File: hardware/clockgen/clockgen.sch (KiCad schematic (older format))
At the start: 2 parts

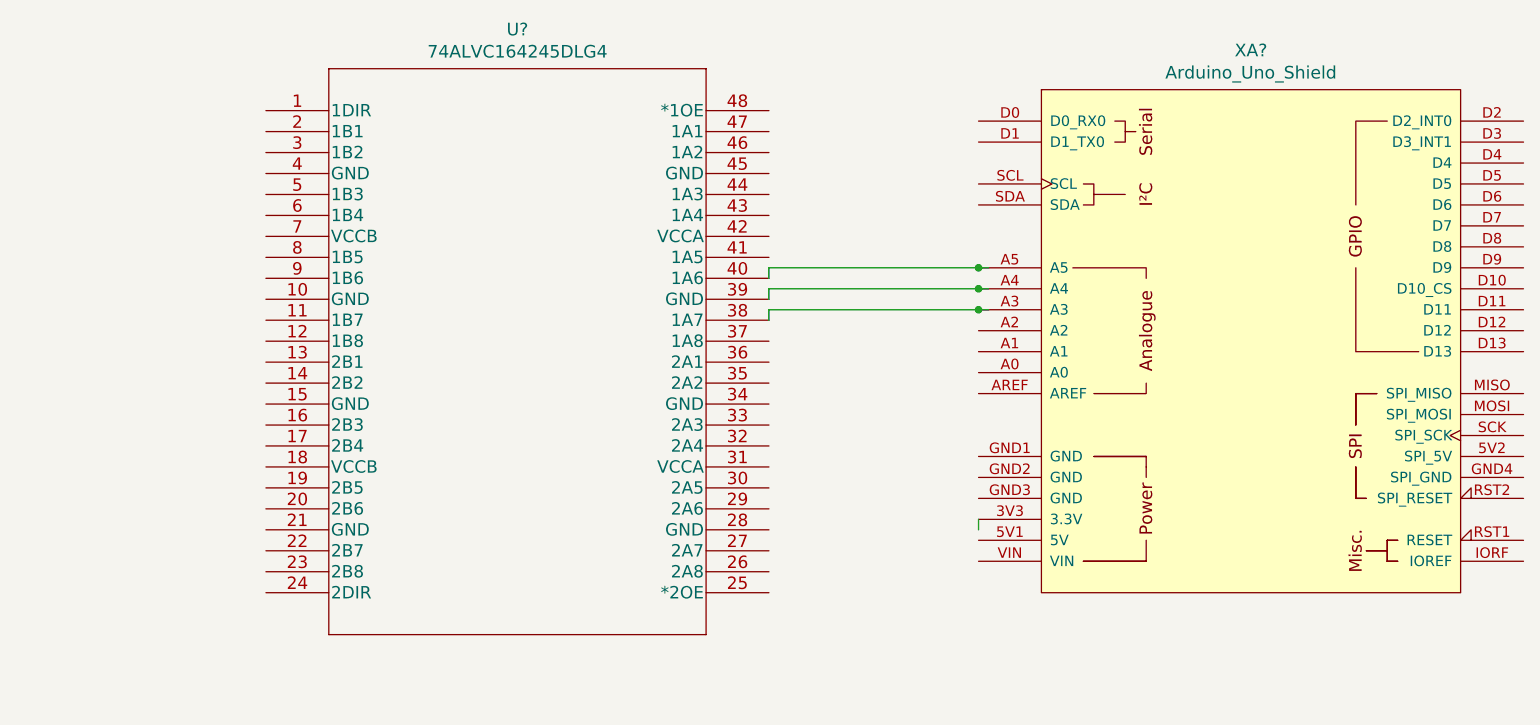
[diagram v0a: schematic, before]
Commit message: Working on PCB
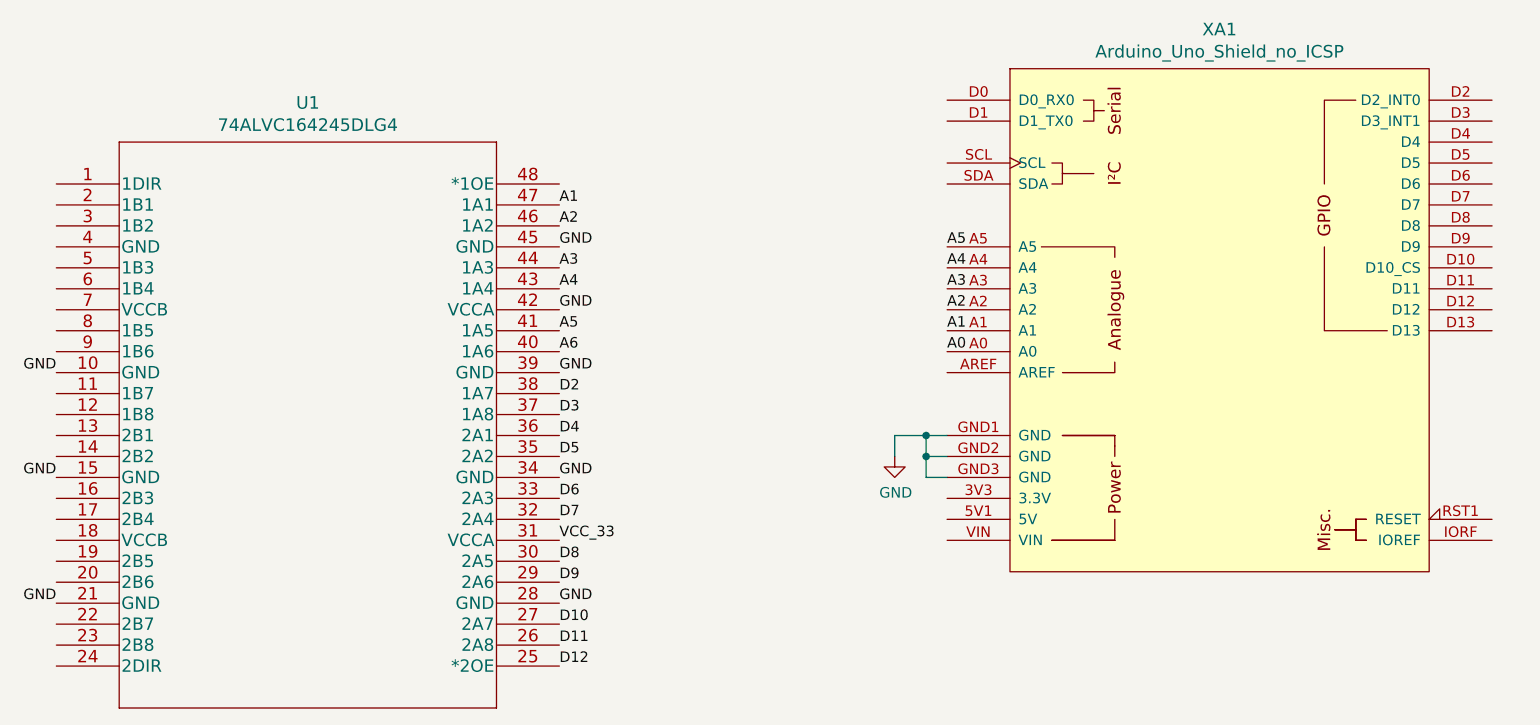
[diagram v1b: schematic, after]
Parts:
- removed XA?: Arduino_Uno_Shield, symbol arduino:Arduino_Uno_Shield
- added XA1: Arduino_Uno_Shield_no_ICSP, Arduino:Arduino_Uno_Connector, symbol arduino:Arduino_Uno_Shield_no_ICSP
- U1: renamed from U?; footprint DL48 -> footprints:74ALVC164245DLG4
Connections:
- net labels added: A0, A1, A2, A3, A4, A5, A6, D10, D11, D12, D2, D3, D4, D5, D6, D7, D8, D9, GND, VCC_33
- wire segments 10 -> 7
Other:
- moved on the sheet: U1
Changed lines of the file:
@@
 $EndDescr
 $Comp
-L 2021-08-26_08-32-07:74ALVC164245DLG4 U?
+L 2021-08-26_08-32-07:74ALVC164245DLG4 U1
 U 1 1 61275A01
-P 4000 2750
-F 0 "U?" H 5200 3137 60  0000 C CNN
-F 1 "74ALVC164245DLG4" H 5200 3031 60  0000 C CNN
-F 2 "DL48" H 5200 2990 60  0001 C CNN
-F 3 "" H 4000 2750 60  0000 C CNN
-	1    4000 2750
+P 3000 3100
+F 0 "U1" H 4200 3487 60  0000 C CNN
+F 1 "74ALVC164245DLG4" H 4200 3381 60  0000 C CNN
+F 2 "footprints:74ALVC164245DLG4" H 4200 3340 60  0001 C CNN
+F 3 "" H 3000 3100 60  0000 C CNN
+	1    3000 3100
+	1    0    0    -1
+$EndComp
+Text Label 5400 3200 0    50   ~ 0
+A1
+Text Label 5400 3300 0    50   ~ 0
+A2
+Text Label 7250 3400 0    50   ~ 0
+A5
+Text Label 7250 3500 0    50   ~ 0
+A4
+Text Label 5400 3500 0    50   ~ 0
+A3
+Text Label 5400 3600 0    50   ~ 0
+A4
+Text Label 5400 3800 0    50   ~ 0
+A5
+Text Label 5400 3900 0    50   ~ 0
+A6
+Text Label 7250 3600 0    50   ~ 0
+A3
+Text Label 7250 3700 0    50   ~ 0
+A2
+Text Label 7250 3800 0    50   ~ 0
+A1
+Text Label 7250 3900 0    50   ~ 0
+A0
+Text Label 5400 3400 0    50   ~ 0
+GND
+Text Label 5400 3700 0    50   ~ 0
+GND
+Text Label 5400 4000 0    50   ~ 0
+GND
+$Comp
+L power:GND #PWR0101
+U 1 1 612D9330
+P 7000 4400
+F 0 "#PWR0101" H 7000 4150 50  0001 C CNN
+F 1 "GND" H 7005 4227 50  0000 C CNN
+F 2 "" H 7000 4400 50  0001 C CNN
+F 3 "" H 7000 4400 50  0001 C CNN
+	1    7000 4400
+	1    0    0    -1
+$EndComp
+$Comp
+L arduino:Arduino_Uno_Shield_no_ICSP XA1
+U 1 1 61298011
+P 8550 3750
+F 0 "XA1" H 8550 5137 60  0000 C CNN
+F 1 "Arduino_Uno_Shield_no_ICSP" H 8550 5031 60  0000 C CNN
+F 2 "Arduino:Arduino_Uno_Connector" H 10350 7500 60  0001 C CNN
+F 3 "https://store.arduino.cc/arduino-uno-rev3" H 10350 7500 60  0001 C CNN
+	1    8550 3750
 	1    0    0    -1
 $EndComp
 Wire Wire Line
-	7450 3500 7400 3500
+	7250 4300 7150 4300
 Wire Wire Line
-	6400 3500 6400 3550
+	7000 4300 7000 4400
 Wire Wire Line
-	7450 3600 7400 3600
+	7250 4400 7150 4400
 Wire Wire Line
-	6400 3600 6400 3650
+	7150 4400 7150 4300
+Connection ~ 7150 4300
 Wire Wire Line
-	7450 3700 7400 3700
+	7150 4300 7000 4300
 Wire Wire Line
-	6400 3700 6400 3750
+	7250 4500 7150 4500
 Wire Wire Line
-	7400 4750 7400 4700
-$Comp
-L arduino:Arduino_Uno_Shield XA?
-U 1 1 61277613
-P 8700 3850
-F 0 "XA?" H 8700 5237 60  0000 C CNN
-F 1 "Arduino_Uno_Shield" H 8700 5131 60  0000 C CNN
-F 2 "" H 10500 7600 60  0001 C CNN
-F 3 "https://store.arduino.cc/arduino-uno-rev3" H 10500 7600 60  0001 C CNN
-	1    8700 3850
-	1    0    0    -1
-$EndComp
-Connection ~ 7400 3500
-Wire Wire Line
-	7400 3500 6400 3500
-Connection ~ 7400 3600
-Wire Wire Line
-	7400 3600 6400 3600
-Connection ~ 7400 3700
-Wire Wire Line
-	7400 3700 6400 3700
+	7150 4500 7150 4400
+Connection ~ 7150 4400
+Text Label 3000 4000 2    50   ~ 0
+GND
+Text Label 3000 4500 2    50   ~ 0
+GND
+Text Label 3000 5100 2    50   ~ 0
+GND
+Text Label 5400 4100 0    50   ~ 0
+D2
+Text Label 5400 4200 0    50   ~ 0
+D3
+Text Label 5400 4300 0    50   ~ 0
+D4
+Text Label 5400 4400 0    50   ~ 0
+D5
+Text Label 5400 4600 0    50   ~ 0
+D6
+Text Label 5400 4700 0    50   ~ 0
+D7
+Text Label 5400 4500 0    50   ~ 0
+GND
+Text Label 5400 4800 0    50   ~ 0
+VCC_33
+Text Label 5400 4900 0    50   ~ 0
+D8
+Text Label 5400 5000 0    50   ~ 0
+D9
+Text Label 5400 5200 0    50   ~ 0
+D10
+Text Label 5400 5300 0    50   ~ 0
+D11
+Text Label 5400 5400 0    50   ~ 0
+D12
+Text Label 5400 5100 0    50   ~ 0
+GND
 $EndSCHEMATC
